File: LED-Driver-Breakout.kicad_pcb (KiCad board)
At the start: 6 copper layers, 98 x 100 mm, 17 parts, among them J1 S2B-XH-A, J2 LED Output, J3 XT60, J4 01x03_PinHeaderSwitch, U1 V10P45-M3/86A, U2 TSR2-24120

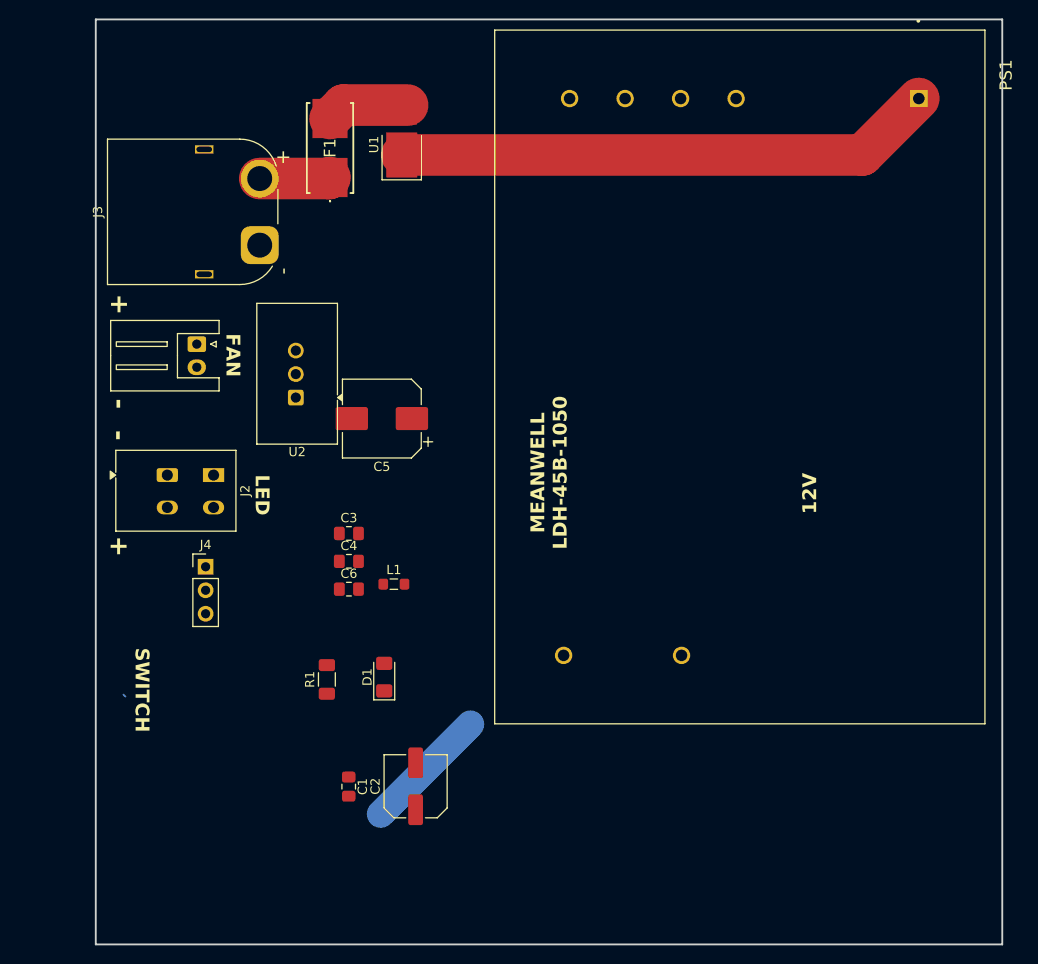
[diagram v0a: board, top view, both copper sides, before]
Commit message: did layout, still need to fix ERC errors and DRC warnings
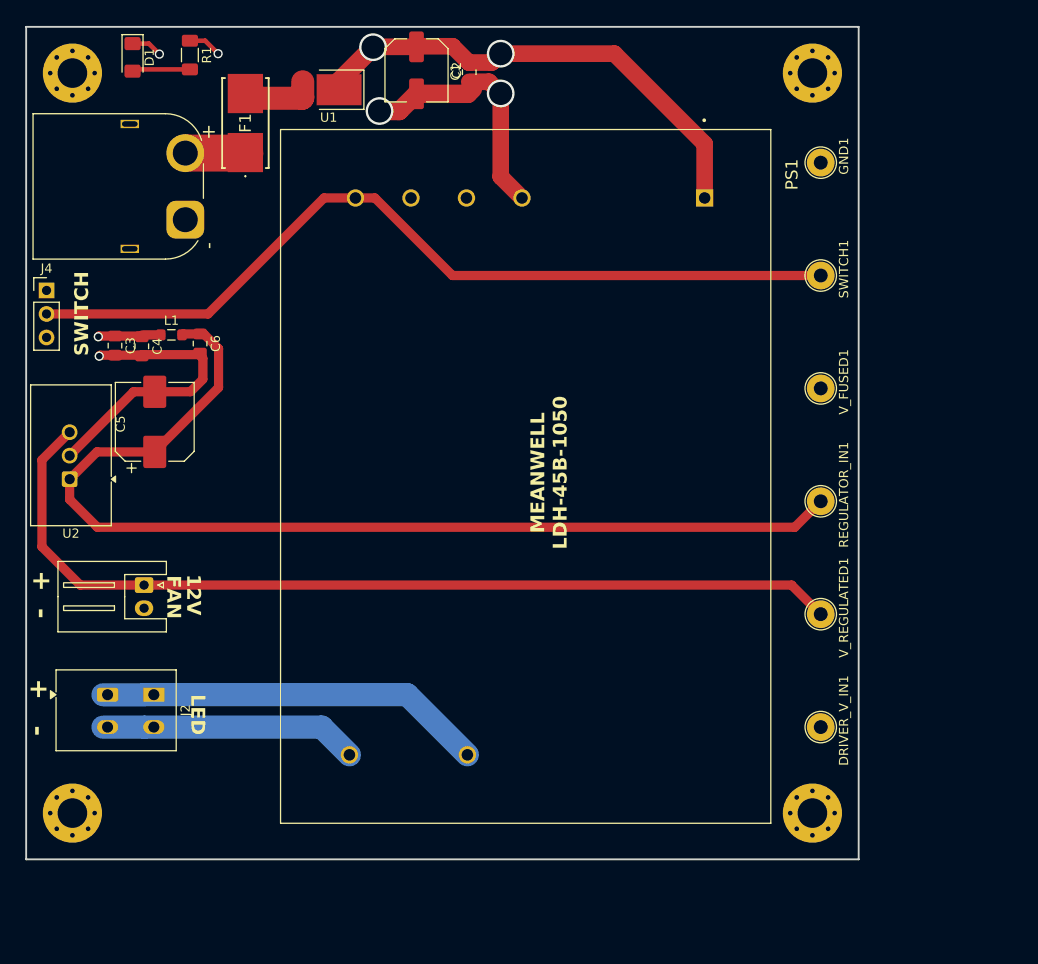
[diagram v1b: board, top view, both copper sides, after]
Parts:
- added DRIVER_V_IN1: TestPoint, TestPoint:TestPoint_Loop_D2.54mm_Drill1.5mm_Beaded, F.Cu at (145.9, 125.7)
- added GND: MountingHole_3.2mm_M3_Pad_Via, MountingHole:MountingHole_3.2mm_M3_Pad_Via, F.Cu at (145.0, 135.0)
- added GND1: TestPoint, TestPoint:TestPoint_Loop_D2.54mm_Drill1.5mm_Beaded, F.Cu at (145.9, 64.7)
- added REF**: MountingHole_3.2mm_M3_Pad_Via, MountingHole:MountingHole_3.2mm_M3_Pad_Via, F.Cu at (65.0, 55.0)
- added REF**: MountingHole_3.2mm_M3_Pad_Via, MountingHole:MountingHole_3.2mm_M3_Pad_Via, F.Cu at (145.0, 55.0)
- added REF**: MountingHole_3.2mm_M3_Pad_Via, MountingHole:MountingHole_3.2mm_M3_Pad_Via, F.Cu at (65.0, 135.0)
- added REGULATOR_IN1: TestPoint, TestPoint:TestPoint_Loop_D2.54mm_Drill1.5mm_Beaded, F.Cu at (145.9, 101.3)
- added SWITCH1: TestPoint, TestPoint:TestPoint_Loop_D2.54mm_Drill1.5mm_Beaded, F.Cu at (145.9, 76.9)
- added V_FUSED1: TestPoint, TestPoint:TestPoint_Loop_D2.54mm_Drill1.5mm_Beaded, F.Cu at (145.9, 89.1)
- added V_REGULATED1: TestPoint, TestPoint:TestPoint_Loop_D2.54mm_Drill1.5mm_Beaded, F.Cu at (145.9, 113.5)
- moved C1 78.3 mm to (107.9, 54.9), turned to -90 degrees
- moved C2 77.4 mm to (102.2, 54.7), turned to -90 degrees
- moved D1 72.3 mm to (71.5, 53.3), turned to -90 degrees
- moved R1 69.1 mm to (77.7, 53.0), turned to -90 degrees
- moved L1 36.1 mm to (75.7, 83.3)
- moved J4 34.5 mm to (62.2, 78.5)
- moved C3 32.4 mm to (69.6, 84.5), turned to -90 degrees
- moved C4 32.3 mm to (72.5, 84.5), turned to -90 degrees
- moved C6 31.0 mm to (78.8, 84.2), turned to -90 degrees
- moved J1 26.7 mm to (72.7, 110.3)
- moved U2 26.0 mm to (64.7, 98.9)
- moved PS1 25.5 mm to (114.0, 98.6)
- moved J2 24.6 mm to (68.8, 122.2)
- moved C5 24.6 mm to (73.9, 92.7), turned to 90 degrees
- moved U1 9.88 mm to (92.7, 56.8), turned to 180 degrees
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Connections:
- net /V_Fused renamed +24V
- net /switch renamed /SWITCH
- net Net-(U2-Vin) renamed /REGULATOR_V_IN
- net Net-(U2-Vout) renamed /V_REGULATED
- C1 pad 2: Net-(PS1-VIN-) -> /GND
- C2 pad 2: Net-(PS1-VIN-) -> /GND
- C3 pad 2: Net-(U2-GND) -> /GND
- C4 pad 2: Net-(U2-GND) -> /GND
- C5 pad 2: Net-(U2-GND) -> /GND
- C6 pad 2: Net-(U2-GND) -> /GND
- J3 pad 1: /GND -> Net-(J3-Pad1)
- J4 pad 1: /GND -> Net-(J4-Pin_1)
- PS1 pad 2: Net-(PS1-VIN-) -> /GND
- PS1 pad 3: /GND -> Net-(PS1-DIM-)
- U2 pad 2: Net-(U2-GND) -> /GND
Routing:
- net /REGULATOR_V_IN: track 0.00 -> 115.3 mm
- net /V_REGULATED: track 0.00 -> 100.8 mm
- net /SWITCH: track 0.00 -> 92.4 mm
- net /GND: track 0.00 -> 62.3 mm, vias 0 -> 4
- net Net-(PS1-VOUT+): track 13.7 -> 42.1 mm
- net Net-(PS1-VOUT-): track 0.00 -> 27.9 mm
- net Net-(D1-A): track 0.00 -> 6.28 mm
- net +24V: track 58.5 -> 63.5 mm, vias 0 -> 4
- net Net-(F1-Pad1): track 7.65 -> 6.52 mm
- net Net-(F1-Pad2): track 8.99 -> 8.15 mm
- added copper zone on In1.Cu, net +24V
- added copper zone on In2.Cu, net /GND
- removed copper zone on In2.Cu, net +24V
- removed copper zone on In1.Cu, net /GND
- removed copper zone on In4.Cu, net /GND
- removed copper zone on In3.Cu, net /V_REGULATED
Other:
- board size 98 x 100 mm -> 90 x 90 mm
- copper layers 6 -> 4
